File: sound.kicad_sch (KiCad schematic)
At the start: 27 parts, among them P15 AUDIO, P43 CHAN_MIX, P51 JOYSTICK0, P52 JOYSTICK1, U34 74LS393, U48 AY-3-8910, U49 74LS07N, U5 74LS02, U51 STEREO_JACK, U66 74LS157, U67 74LS157

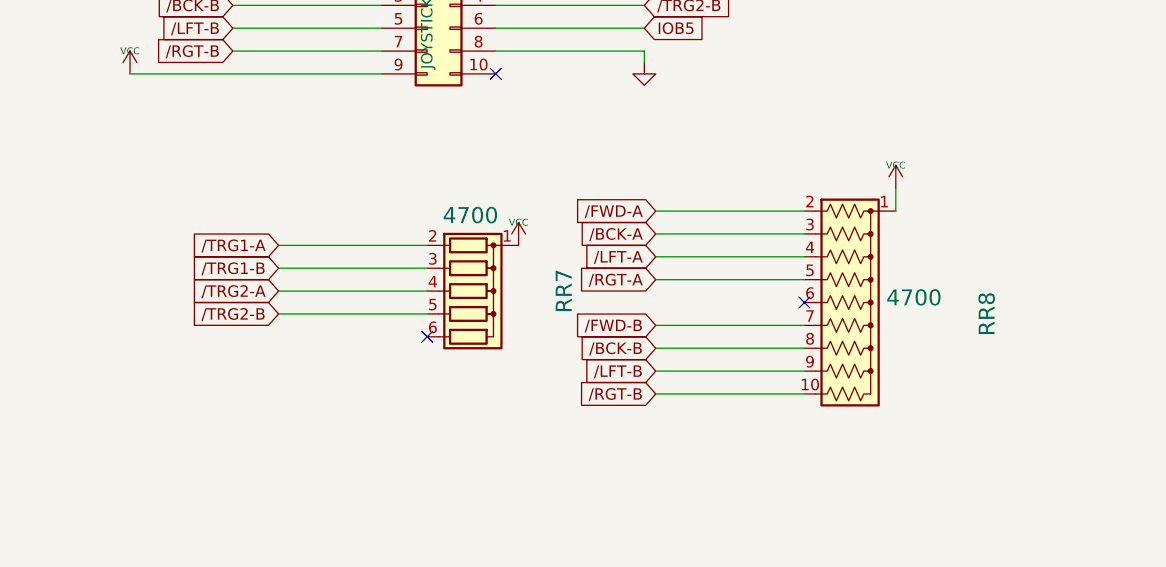
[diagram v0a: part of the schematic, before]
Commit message: rev 1.0
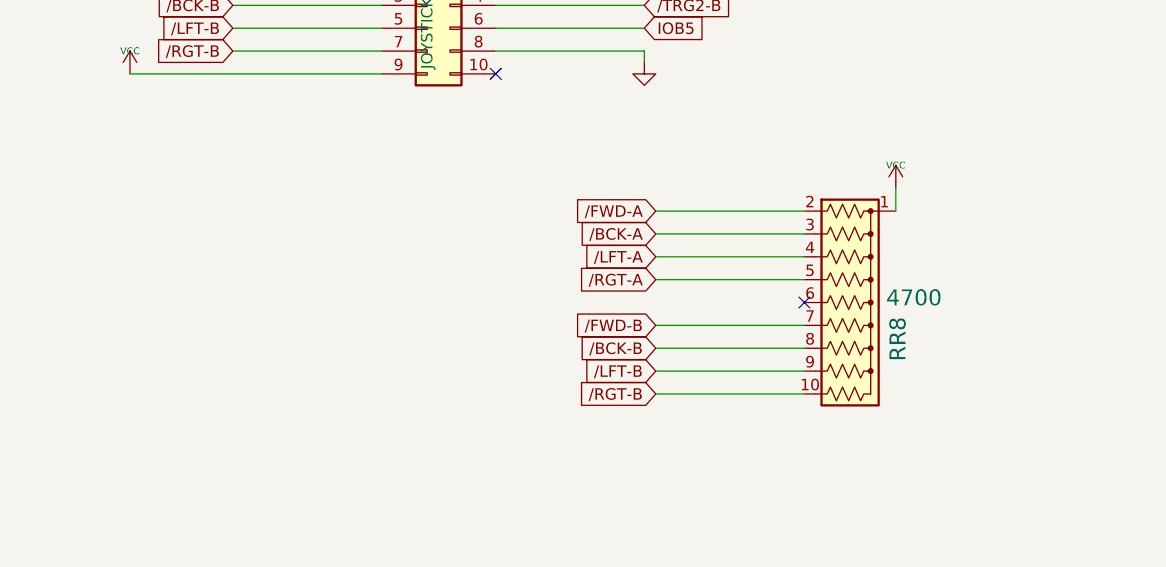
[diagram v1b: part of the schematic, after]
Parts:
- removed RR7: 4700, Resistor_THT:R_Array_SIP6, symbol Device:R_Network05
- RR8: footprint Resistor_THT:R_Array_SIP10 -> Custom:STD_DDW_SIP10
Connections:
- no-connect marks 18 -> 17
